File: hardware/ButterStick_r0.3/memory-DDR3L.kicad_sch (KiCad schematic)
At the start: 0 parts

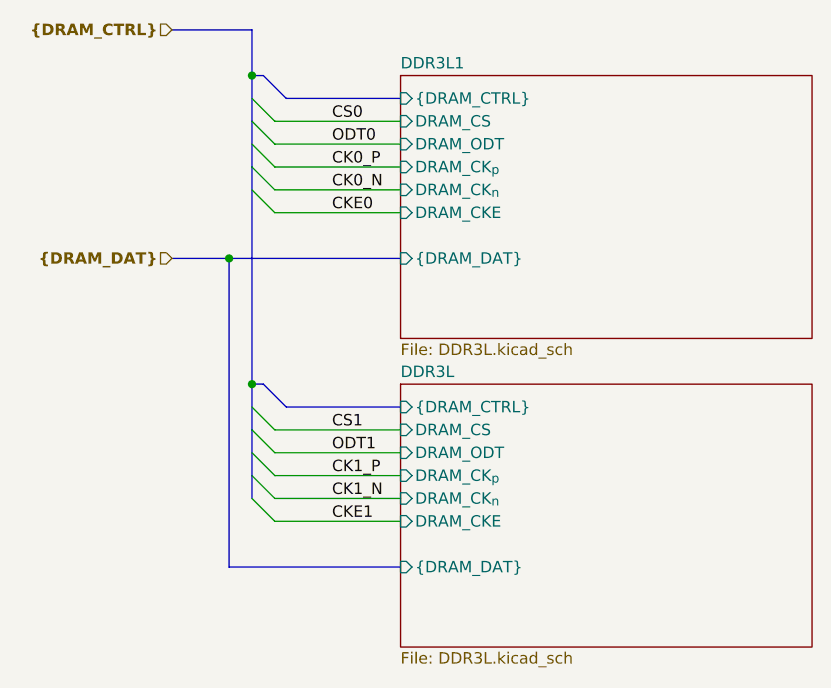
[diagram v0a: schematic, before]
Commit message: hw.r0_3: major blocks roughly routed
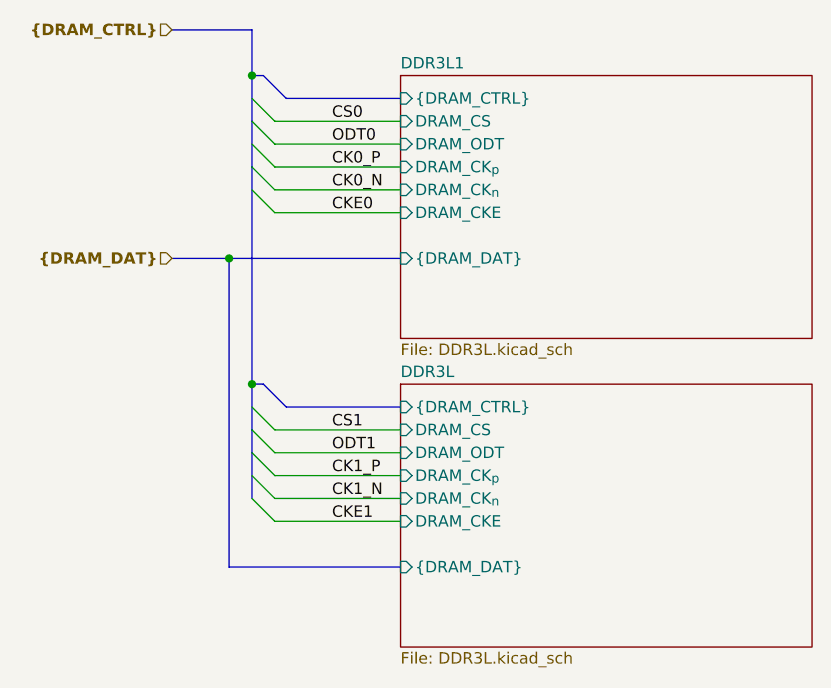
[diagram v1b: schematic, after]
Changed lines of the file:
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@@
   (bus (pts (xy 95.25 99.06) (xy 95.25 104.14)))
   (bus (pts (xy 95.25 99.06) (xy 96.52 99.06)))
-  (bus (pts (xy 95.25 104.14) (xy 95.25 109.22)))
-  (bus (pts (xy 95.25 109.22) (xy 95.25 111.76)))
+  (bus (pts (xy 95.25 104.14) (xy 95.25 106.68)))
+  (bus (pts (xy 95.25 106.68) (xy 95.25 111.76)))
   (bus (pts (xy 96.52 64.77) (xy 99.06 67.31)))
   (bus (pts (xy 99.06 67.31) (xy 111.76 67.31)))
